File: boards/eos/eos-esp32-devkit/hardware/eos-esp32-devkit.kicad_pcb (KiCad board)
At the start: 2 copper layers, 27.9 x 48.8 mm, 36 parts, among them J1 USB-C, J2 J2, J3 J3, Q1 MMBT3904, Q2 MMBT3904, SW1 EN, SW2 BOOT, U1 ESP32-WROOM-32E-N4, U2 SP0503BAHTG, U3 AP7361C-33, U4 CP2102N-A02-GQFN24

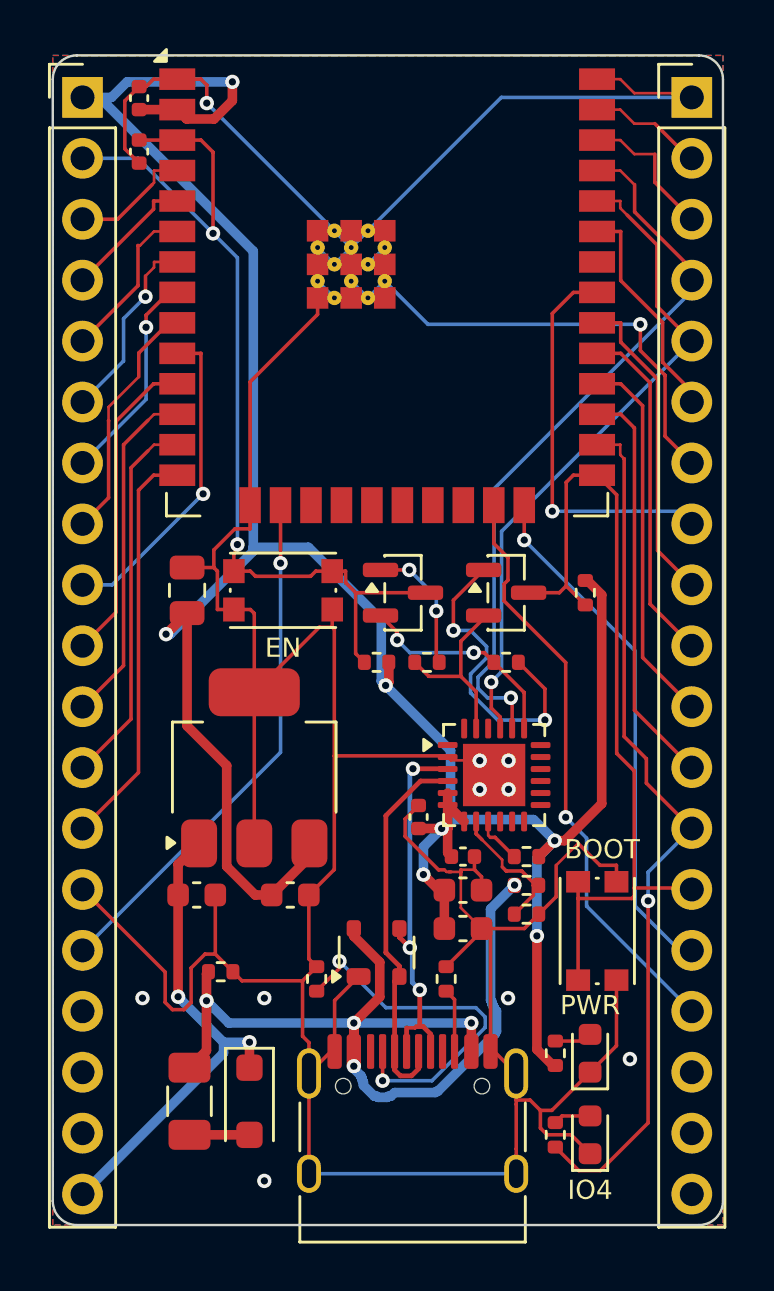
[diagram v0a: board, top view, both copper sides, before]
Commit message: fix(boards): rebuild EoS boards without vias in pads
Co-authored-by: Cursor <cursoragent@cursor.com>
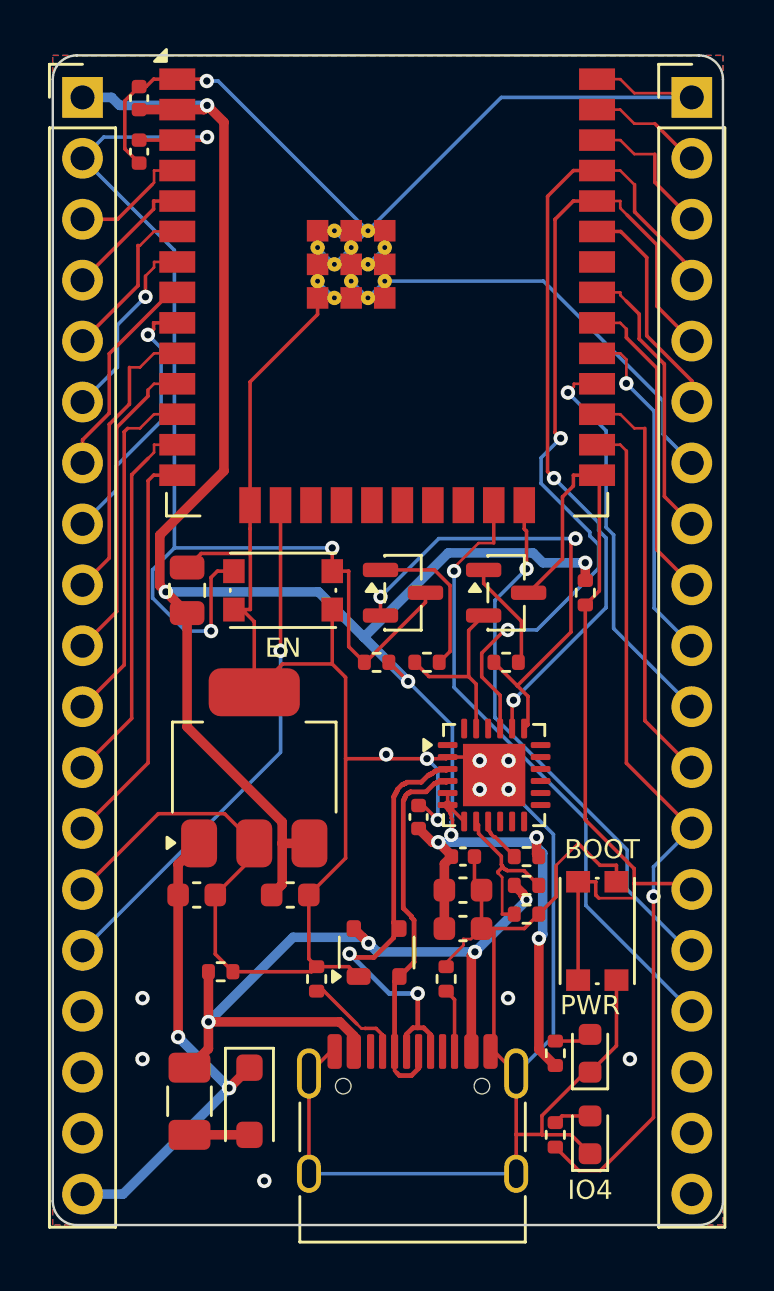
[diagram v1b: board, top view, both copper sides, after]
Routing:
- net /EN: track 39.8 -> 51.3 mm, vias 2 -> 3
- net /RTS: track 9.04 -> 20.5 mm
- net /CC1: track 15.5 -> 4.20 mm, vias 2 -> 0
- net +3V3: track 111.5 -> 100.3 mm, vias 7 -> 8
- net /QB2: track 13.4 -> 4.55 mm, vias 2 -> 0
- net /U0RXD: track 27.8 -> 35.9 mm, vias 1 -> 2
- net VBUS: track 39.3 -> 33.1 mm, vias 5 -> 4
- net /IO19: track 16.5 -> 11.9 mm, vias 1 -> 0
- net /U0TXD: track 30.3 -> 34.1 mm, vias 1 -> 2
- net /USB_D+: track 16.3 -> 18.9 mm, vias 3 -> 2
- net /IO15: track 24.6 -> 26.3 mm
- net /IO25: track 13.5 -> 12.1 mm, vias 1 -> 0
- net /VBUS_SENSE: track 5.78 -> 6.80 mm
- net /IO17: track 15.7 -> 16.7 mm, vias 0 -> 1
- net /QB1: track 5.57 -> 6.56 mm, vias 2 -> 0
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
